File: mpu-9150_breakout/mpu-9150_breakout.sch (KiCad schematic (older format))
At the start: 1 part

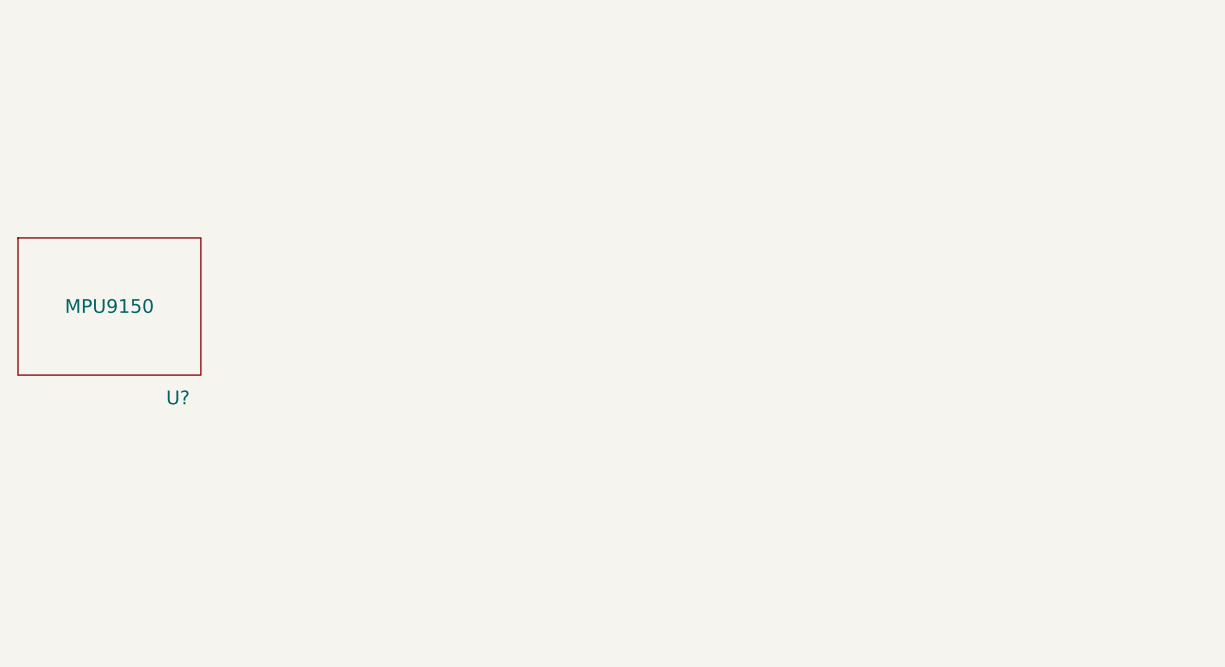
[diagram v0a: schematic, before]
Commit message: Add first pcb layout
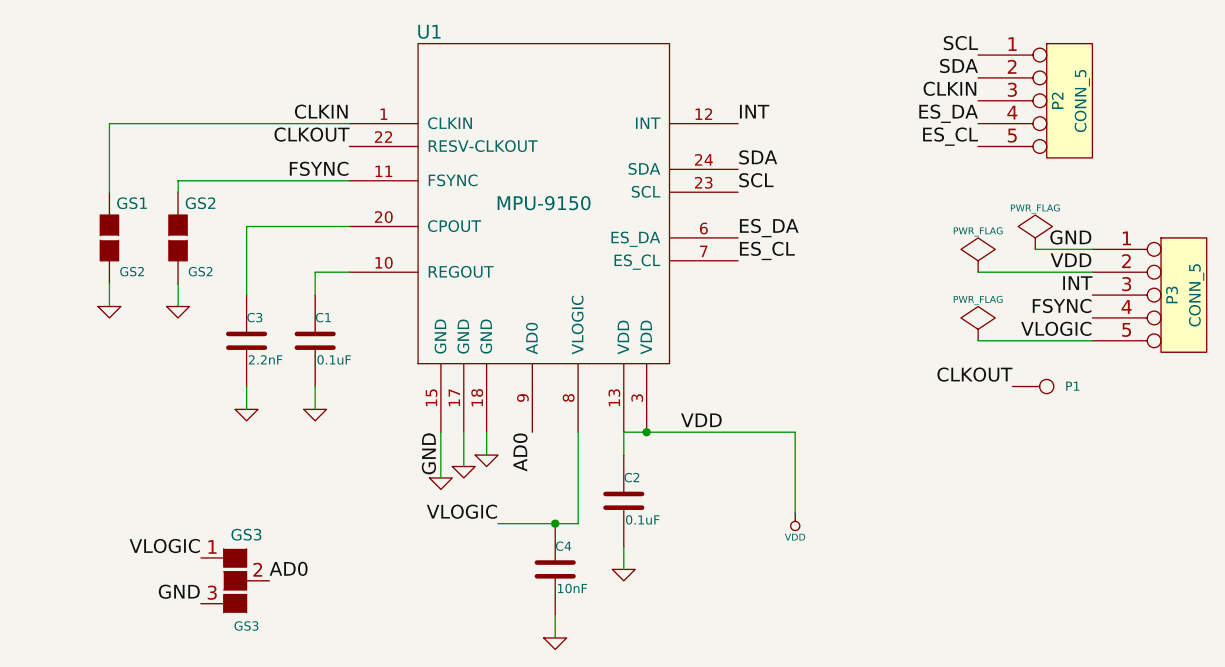
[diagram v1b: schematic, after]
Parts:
- removed U?: MPU9150, symbol MPU9150
- added C1, C2: 0.1uF, ~, symbol C
- added C3: 2.2nF, ~, symbol C
- added C4: 10nF, ~, symbol C
- added GS1, GS2: GS2, ~, symbol GS2
- added GS3: GS3, ~, symbol GS3
- added P1: CONN_1, ~, symbol CONN_1
- added P2, P3: CONN_5, ~, symbol CONN_5
- added U1: MPU-9150, ~, symbol MPU-9150
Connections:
- new net: C1.1, U1.10 (REGOUT)
- new net: C3.1, U1.20 (CPOUT)
- new net AD0: GS3.2 (G2), U1.9 (AD0)
- new net CLKIN: GS1.1 (G1), P2.3, U1.1 (CLKIN)
- new net CLKOUT: P1.1, U1.22 (RESV-CLKOUT)
- new net ES_CL: P2.5, U1.7 (ES_CL)
- new net ES_DA: P2.4, U1.6 (ES_DA)
- new net FSYNC: GS2.1 (G1), P3.4, U1.11 (FSYNC)
- new net GND: C1.2, C2.2, C3.2, C4.2, GS1.2 (G2), GS2.2 (G2), GS3.3 (G3), P3.1, U1.15 (GND), U1.17 (GND), U1.18 (GND)
- new net INT: P3.3, U1.12 (INT)
- new net SCL: P2.1, U1.23 (SCL)
- new net SDA: P2.2, U1.24 (SDA)
- new net VDD: C2.1, P3.2, U1.13 (VDD), U1.3 (VDD)
- new net VLOGIC: C4.1, GS3.1 (G1), P3.5, U1.8 (VLOGIC)
